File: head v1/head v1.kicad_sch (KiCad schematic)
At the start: 5 parts

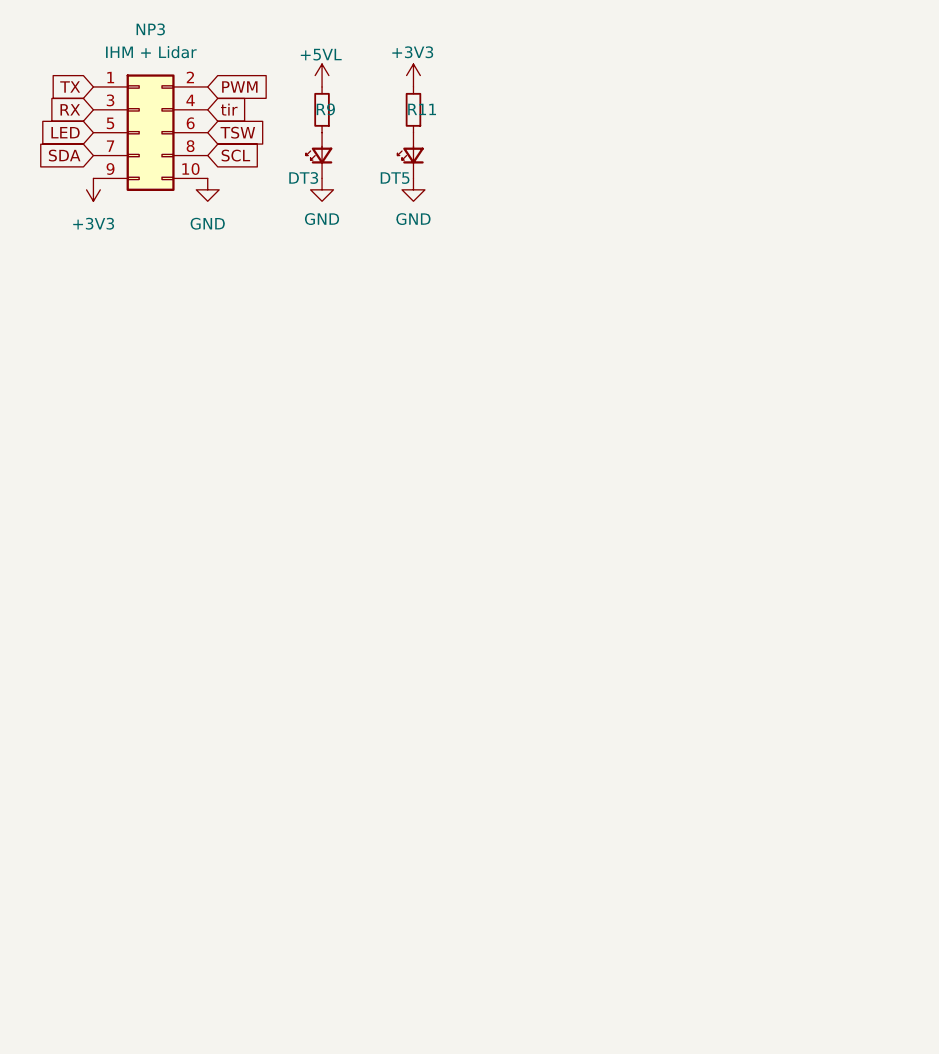
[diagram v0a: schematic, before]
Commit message: head update
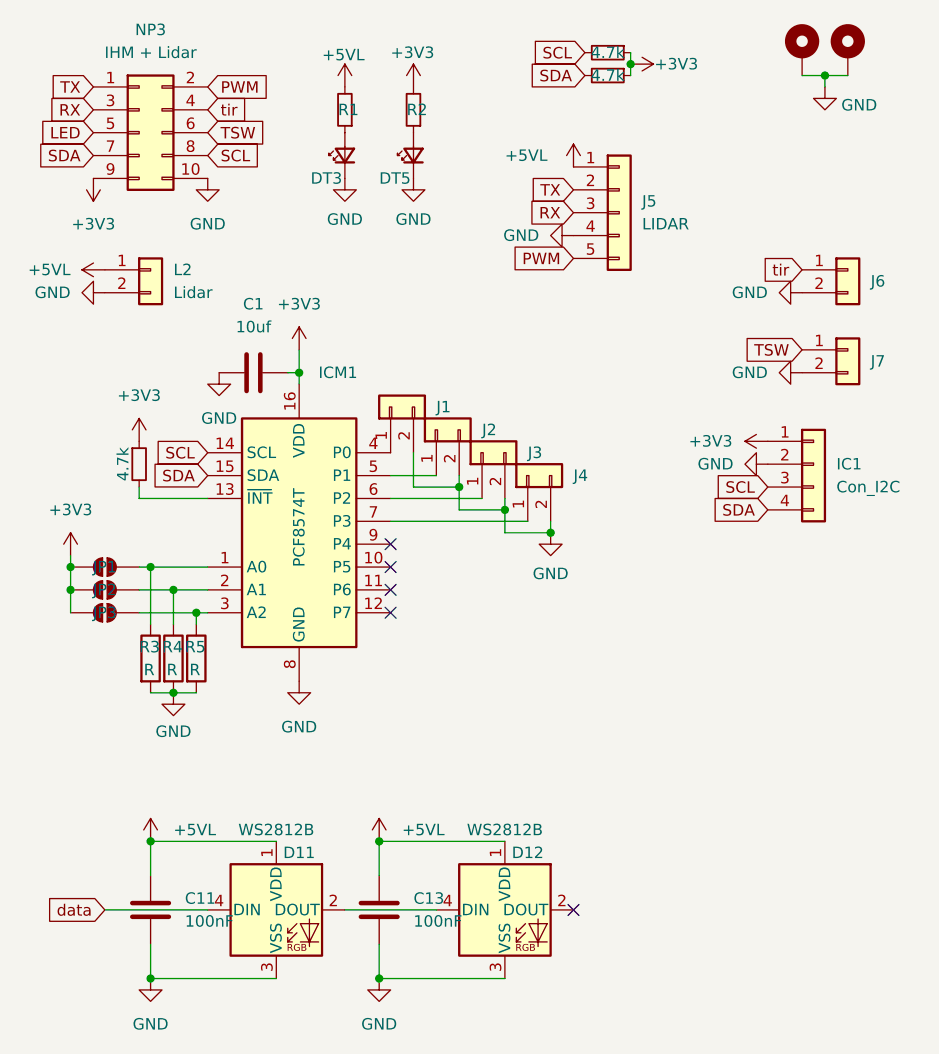
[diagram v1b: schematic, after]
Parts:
- added C1: 10uf, Capacitor_SMD:C_1206_3216Metric_Pad1.33x1.80mm_HandSolder, symbol Device:C
- added C11, C13: 100nF, Capacitor_SMD:C_1206_3216Metric, symbol Device:C
- added D11, D12: WS2812B, LED_SMD:LED_WS2812B_PLCC4_5.0x5.0mm_P3.2mm, symbol LED:WS2812B
- added H1, H2: M3, MountingHole:MountingHole_3.2mm_M3_Pad_Via, symbol Mechanical:MountingHole_Pad
- added IC1: Con_I2C, Connector_Molex:Molex_KK-254_AE-6410-04A_1x04_P2.54mm_Vertical, symbol Connector_Generic:Conn_01x04
- added ICM1: PCF8574T, Package_SO:SOIC-16W_7.5x10.3mm_P1.27mm, symbol Interface_Expansion:PCF8574T
- added J1, J2, J3, J4, J6, J7: Conn_01x02, Connector_Molex:Molex_KK-254_AE-6410-02A_1x02_P2.54mm_Vertical, symbol Connector_Generic:Conn_01x02
- added J5: LIDAR, Connector_JST:JST_XH_B5B-XH-A_1x05_P2.50mm_Vertical, symbol Connector_Generic:Conn_01x05
- added JP1, JP2, JP3: SolderJumper_2_Open, Jumper:SolderJumper-2_P1.3mm_Open_RoundedPad1.0x1.5mm, symbol Jumper:SolderJumper_2_Open
- added L2: Lidar, Connector_Molex:Molex_KK-254_AE-6410-02A_1x02_P2.54mm_Vertical, symbol Connector_Generic:Conn_01x02
- added R3, R4, R5: R, Resistor_SMD:R_1206_3216Metric_Pad1.30x1.75mm_HandSolder, symbol Device:R
- added R6, R7, R8: 4.7k, Resistor_SMD:R_1206_3216Metric_Pad1.30x1.75mm_HandSolder, symbol Device:R_Small
- renumbered R9 to R1, R11 to R2
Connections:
- net +3V3: now also C1.1, IC1.1 (Pin_1), ICM1.16 (VDD), JP1.1 (A), JP2.1 (A), JP3.1 (A), R6.1, R7.1, R8.1
- net +5VL: now also C11.1, C13.1, D11.1 (VDD), D12.1 (VDD), J5.1 (Pin_1), L2.1 (Pin_1)
- net GND: now also C1.2, C11.2, C13.2, D11.3 (VSS), D12.3 (VSS), H1.1, H2.1, IC1.2 (Pin_2), ICM1.8 (GND), J1.2 (Pin_2), J2.2 (Pin_2), J3.2 (Pin_2), J4.2 (Pin_2), J5.4 (Pin_4), J6.2 (Pin_2), J7.2 (Pin_2), L2.2 (Pin_2), R3.2, R4.2, R5.2
- net PWM: now also J5.5 (Pin_5)
- net RX: now also J5.3 (Pin_3)
- net SCL: now also IC1.3 (Pin_3), ICM1.14 (SCL), R7.2
- net SDA: now also IC1.4 (Pin_4), ICM1.15 (SDA), R8.2
- net TSW: now also J7.1 (Pin_1)
- net TX: now also J5.2 (Pin_2)
- net tir: now also J6.1 (Pin_1)
- new net: D11.2 (DOUT), D12.4 (DIN)
- new net: ICM1.6 (P2), J3.1 (Pin_1)
- new net: ICM1.7 (P3), J4.1 (Pin_1)
- new net: ICM1.2 (A1), JP2.2 (B), R4.1
- new net: ICM1.1 (A0), JP1.2 (B), R3.1
- new net: ICM1.13 (~{INT}), R6.2
- new net: ICM1.3 (A2), JP3.2 (B), R5.1
- new net: ICM1.4 (P0), J1.1 (Pin_1)
- new net: ICM1.5 (P1), J2.1 (Pin_1)
- new net data: D11.4 (DIN)
- no-connect marks 0 -> 5
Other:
- moved on the sheet: DT3, R1
